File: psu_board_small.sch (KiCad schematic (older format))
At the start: 40 parts, among them J1 AC1, J10 GND, J11 V-, J12 V-, J2 GND2, J3 GND3, J4 AC4, J5 LED, J6 LED, J7 V+, J8 V+, J9 GND

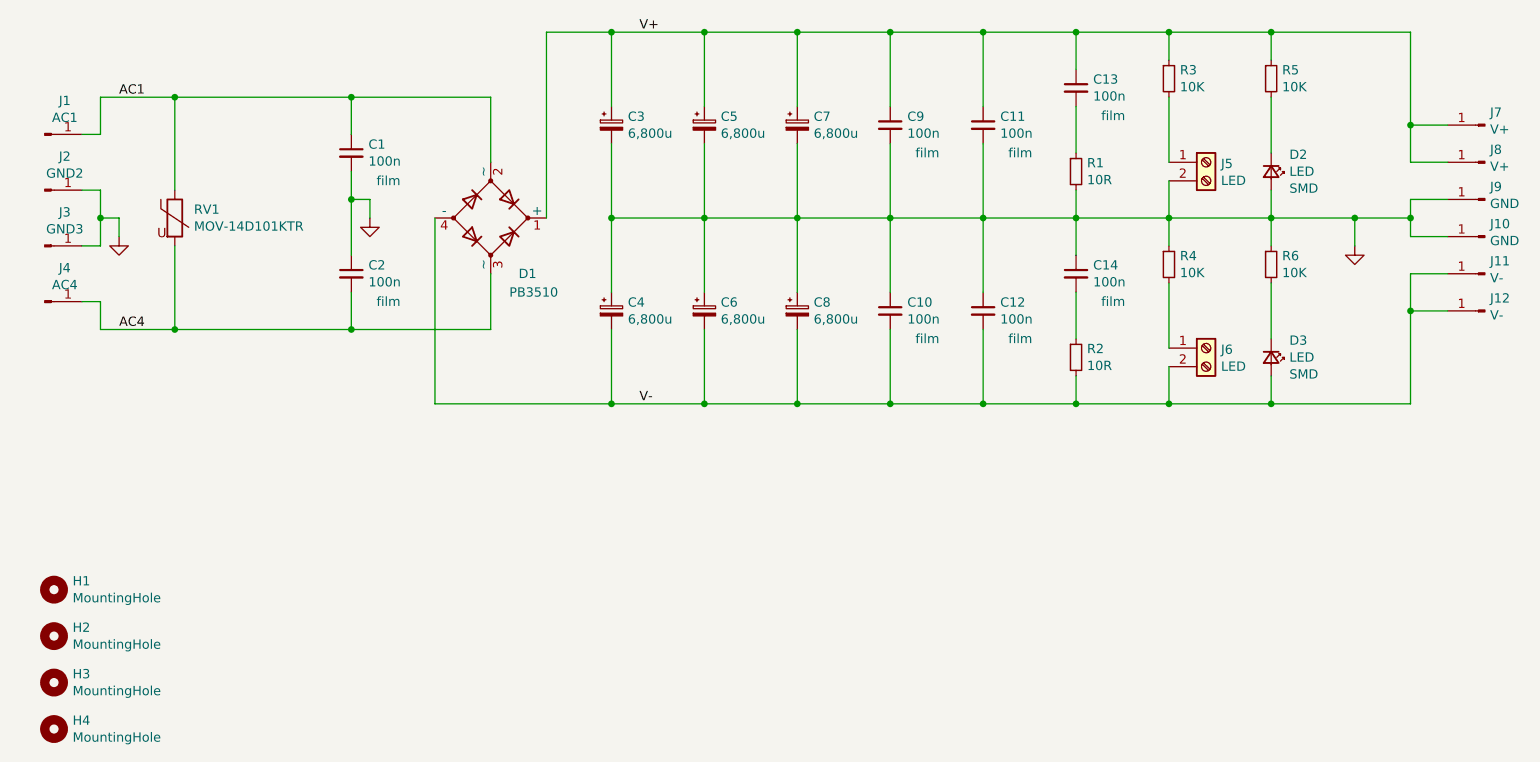
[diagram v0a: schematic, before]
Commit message: finished sch
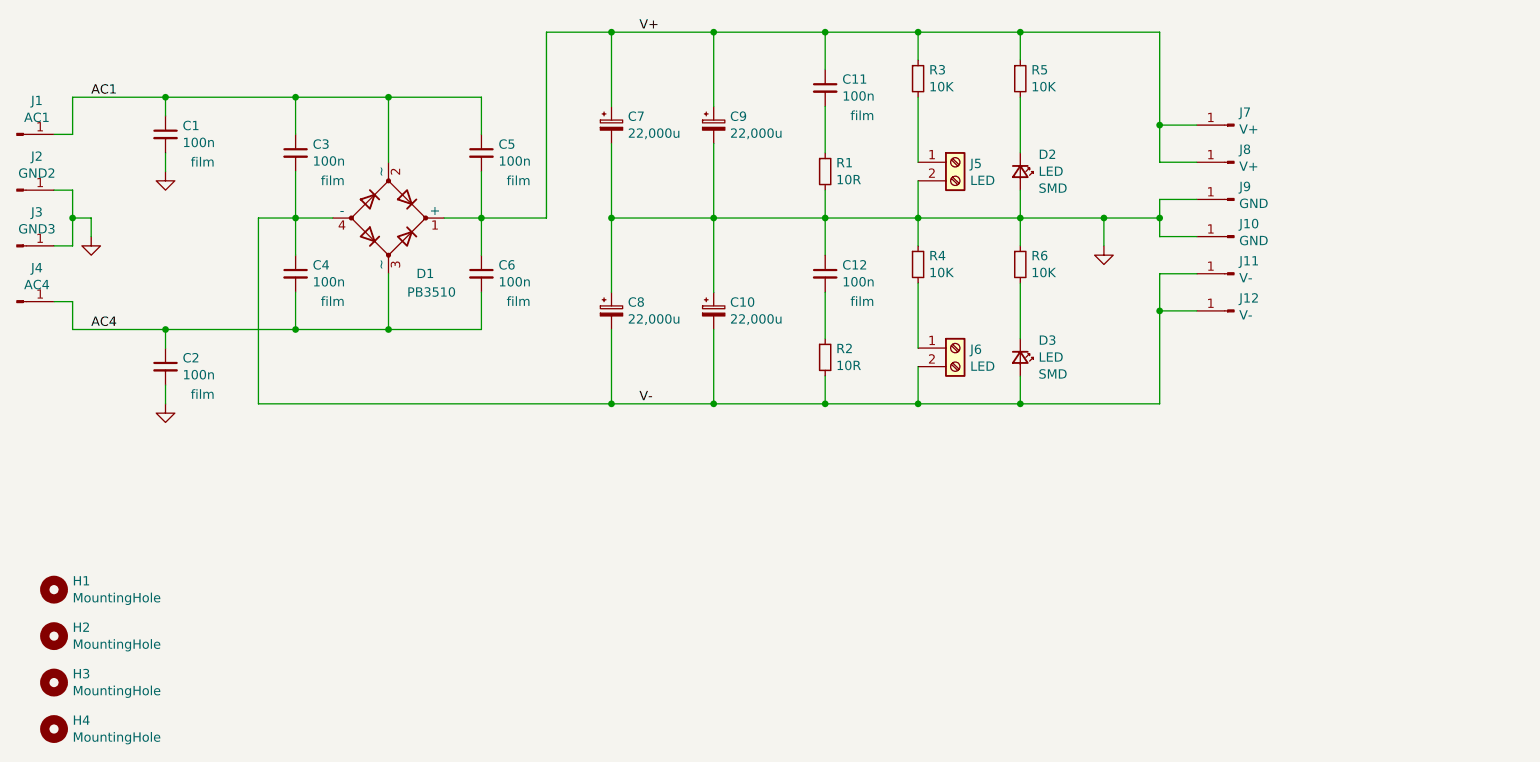
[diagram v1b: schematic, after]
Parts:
- removed C10, C11, C12, C9: 100n, Capacitor_THT:C_Rect_L7.2mm_W2.5mm_P5.00mm_FKS2_FKP2_MKS2_MKP2, symbol Device:C_Small
- removed C7, C8: 6,800u, Capacitor_THT:CP_Radial_D25.0mm_P10.00mm_SnapIn, symbol Device:CP_Small
- removed RV1: MOV-14D101KTR, Varistor:RV_Disc_D15.5mm_W3.9mm_P7.5mm, symbol Device:Varistor
- added C3, C4, C5, C6: 100n, Capacitor_THT:C_Rect_L7.2mm_W2.5mm_P5.00mm_FKS2_FKP2_MKS2_MKP2, symbol Device:C_Small
- C10: renamed from C6; value 6,800u -> 22,000u
- C7: renamed from C3; value 6,800u -> 22,000u
- C8: renamed from C4; value 6,800u -> 22,000u
- C9: renamed from C5; value 6,800u -> 22,000u
- renumbered C13 to C11, C14 to C12
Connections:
- net AC1: now also C3.1, C5.1
- net AC4: now also C2.1, C4.2, C6.2; no longer C2.2
- net GND: now also C2.2; no longer C2.1
- net V+: now also C5.2, C6.1
- net V-: now also C3.2, C4.1
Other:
- moved on the sheet: C1, C10, C11, C12, C2, C9, D1, D2, D3, J1, J10, J11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
